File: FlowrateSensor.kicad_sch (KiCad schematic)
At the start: 4 parts, among them Q3 NMOS

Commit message: Initial layout with 1 pump, 2 temp, 1 flow all on front side
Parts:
- Q3: footprint Package_TO_SOT_SMD:LFPAK33 -> Package_TO_SOT_SMD:SOT-23
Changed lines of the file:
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@@
 			)
 		)
-		(property "Footprint" "Package_TO_SOT_SMD:LFPAK33"
+		(property "Footprint" "Package_TO_SOT_SMD:SOT-23"
 			(at 118.11 41.91 0)
 			(effects

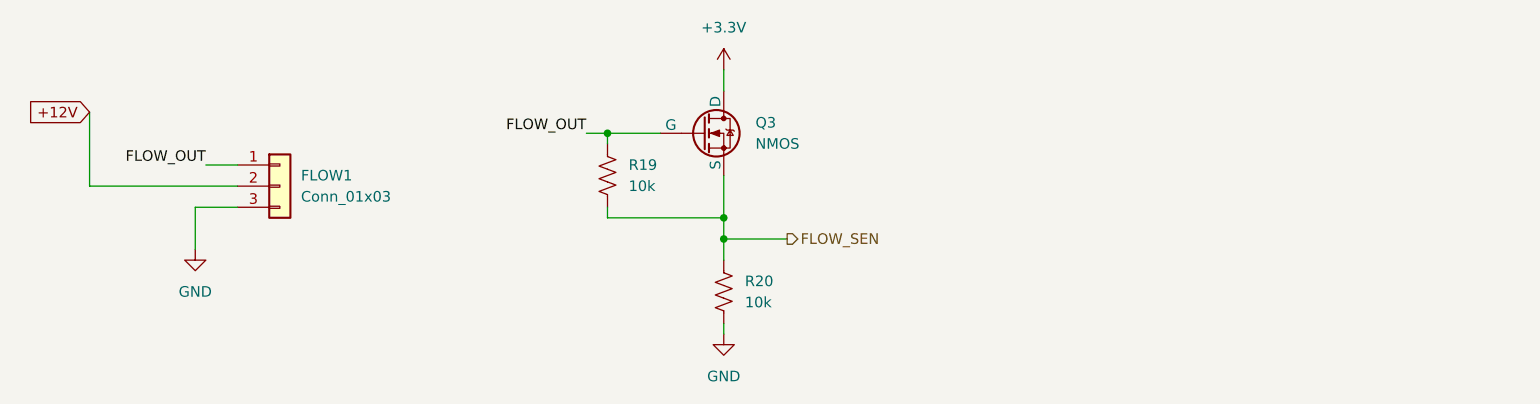
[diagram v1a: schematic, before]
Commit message: schematic with 12V components, unigain buffers & extra temp sensor
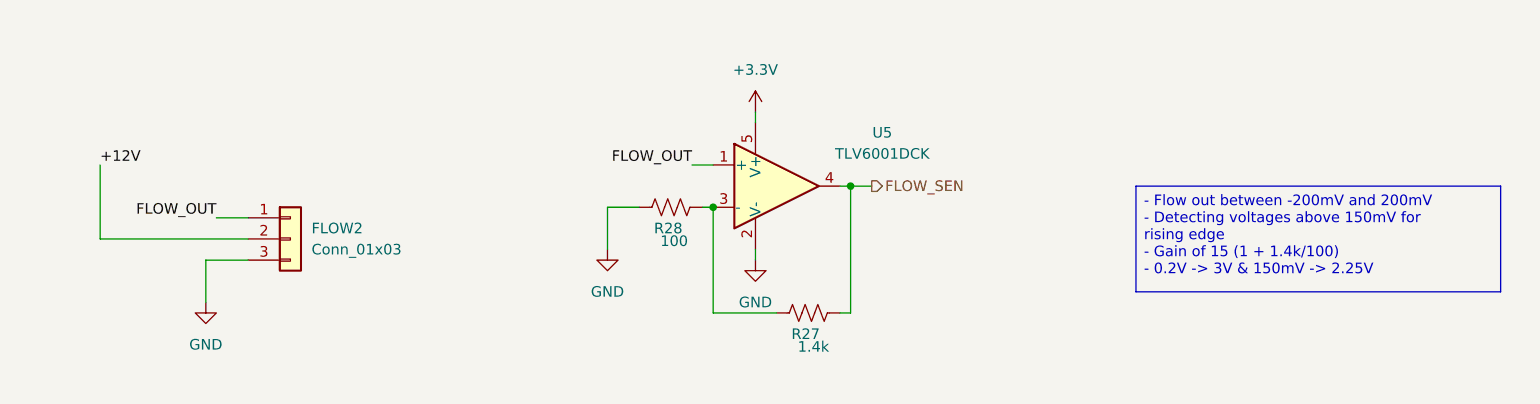
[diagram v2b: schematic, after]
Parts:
- removed FLOW1: Conn_01x03, UTSVT_Connectors:Molex_MicroFit3.0_1x3xP3.00mm_PolarizingPeg_Vertical, symbol Connector_Generic:Conn_01x03
- removed Q3: NMOS, Package_TO_SOT_SMD:SOT-23, symbol Simulation_SPICE:NMOS
- removed R19, R20: 10k, Resistor_SMD:R_0805_2012Metric, symbol Device:R_US
- added FLOW2: Conn_01x03, Connector_Molex:Molex_Nano-Fit_105309-xx03_1x03_P2.50mm_Vertical, symbol Connector_Generic:Conn_01x03
- added R27: 1.4k, Resistor_SMD:R_0805_2012Metric, symbol Device:R_US
- added R28: 100, Resistor_SMD:R_0805_2012Metric, symbol Device:R_US
- added U5: TLV6001DCK, Package_TO_SOT_SMD:SOT-353_SC-70-5, symbol Amplifier_Operational:TLV6001DCK
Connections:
- net +12V: now also FLOW2.2 (Pin_2)
- net +3.3V: now also U5.5 (V+)
- net FLOW_OUT: now also FLOW2.1 (Pin_1), U5.1 (+)
- net FLOW_SEN: now also R27.1, U5.4
- net GND: now also FLOW2.3 (Pin_3), R28.2, U5.2 (V-)
- new net: R27.2, R28.1, U5.3 (-)
